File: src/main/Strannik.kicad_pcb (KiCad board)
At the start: 2 copper layers, 139 x 129 mm, 104 parts, among them J1 Thumb cluster, J2 Battery, SW1 Reset, SW11 SW_Push_Dual, SW12 SW_Push_Dual, SW13 SW_Push_Dual, SW14 SW_Push_Dual, SW15 SW_Push_Dual, SW16 SW_Push_Dual, SW17 SW_Push_Dual, SW21 SW_Push_Dual, SW22 SW_Push_Dual, SW23 SW_Push_Dual, SW24 SW_Push_Dual, SW25 SW_Push_Dual, SW26 SW_Push_Dual, SW27 SW_Push_Dual, SW31 SW_Push_Dual, SW32 SW_Push_Dual, SW33 SW_Push_Dual, SW34 SW_Push_Dual, SW35 SW_Push_Dual, SW36 SW_Push_Dual, SW37 SW_Push_Dual, SW41 SW_Push_Dual, SW42 SW_Push_Dual, SW43 SW_Push_Dual, SW44 SW_Push_Dual, SW45 SW_Push_Dual, SW46 SW_Push_Dual, SW51 SW_Push_Dual, SW52 SW_Push_Dual, SW53 SW_Push_Dual, SW54 SW_Push_Dual, SW55 SW_Push_Dual

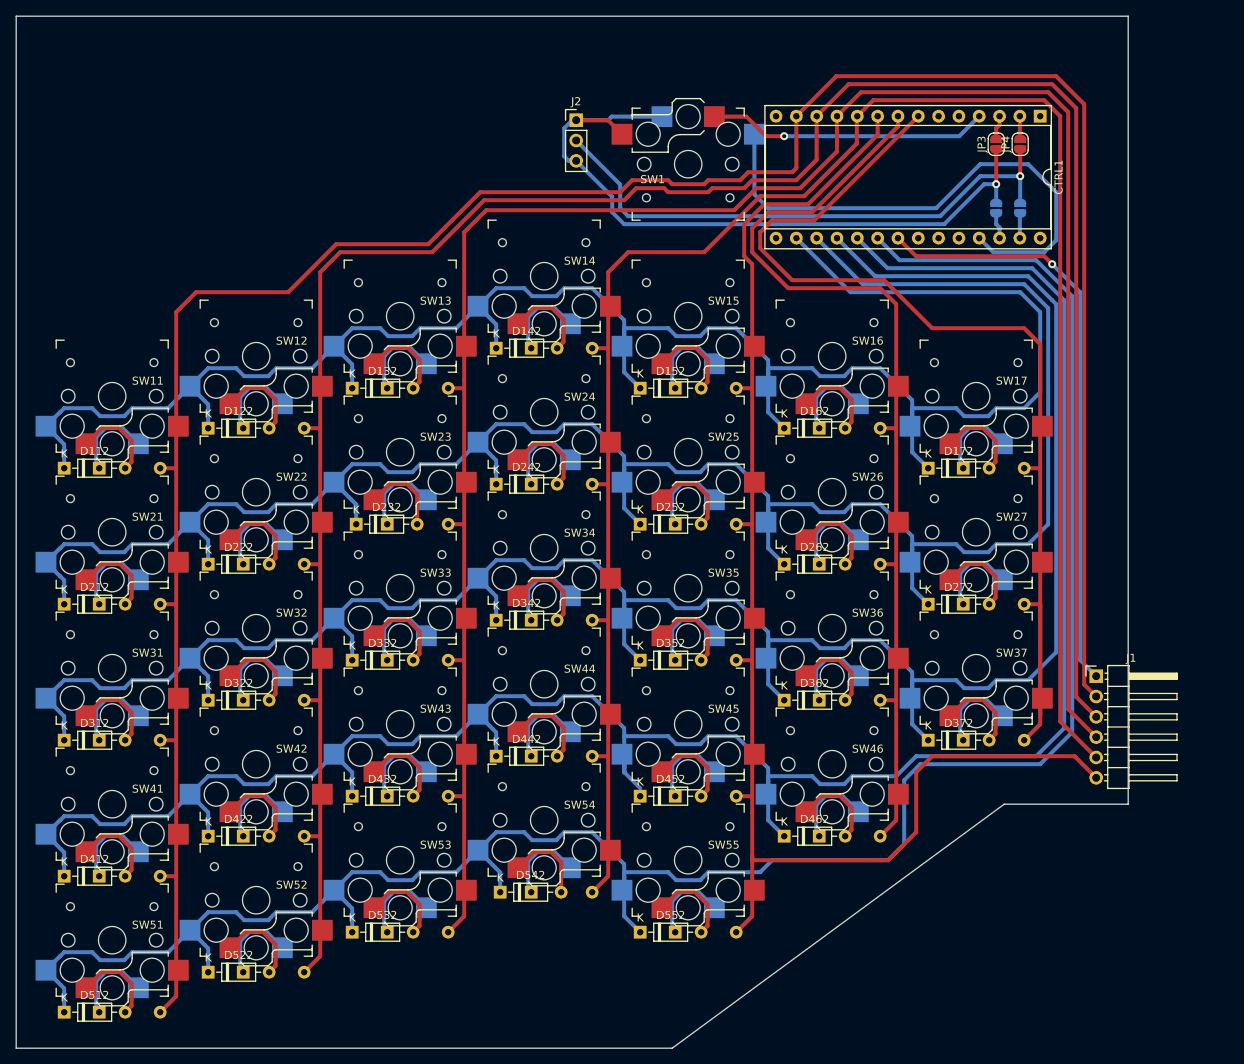
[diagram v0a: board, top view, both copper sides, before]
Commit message: new beautiful main board design
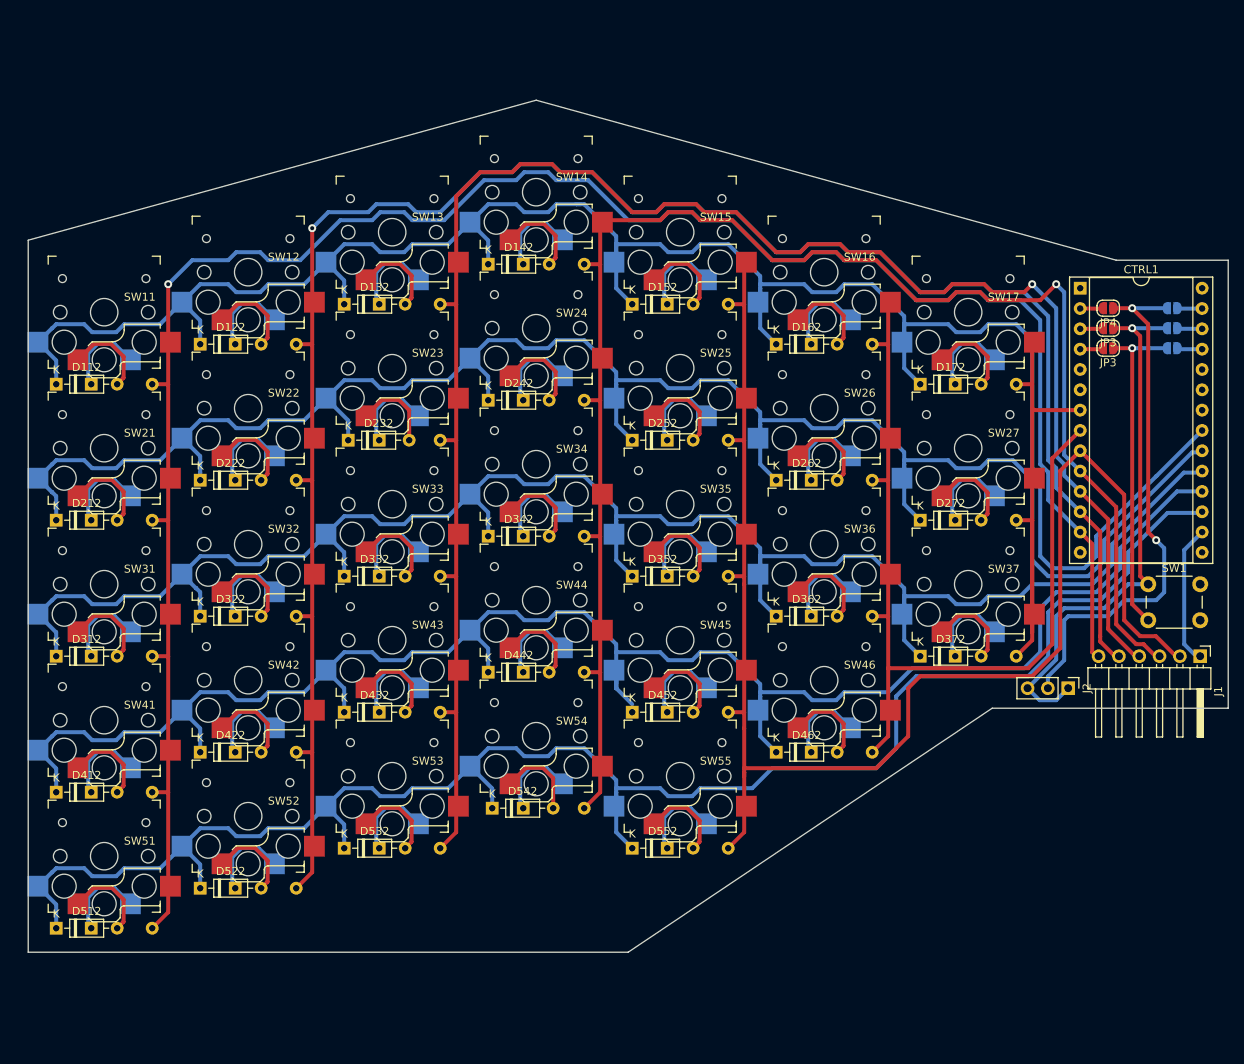
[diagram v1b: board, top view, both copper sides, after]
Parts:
- added JP1: Ground Left, Jumper:SolderJumper-2_P1.3mm_Open_RoundedPad1.0x1.5mm, B.Cu at (189.5, 76.5)
- added JP3: Ground Right, Jumper:SolderJumper-2_P1.3mm_Open_RoundedPad1.0x1.5mm, F.Cu at (181.5, 76.5)
- SW1: footprint Keyswitches:Kailh_socket_PG1350_reversible -> Button_Switch_THT:SW_PUSH_6mm_H4.3mm
- moved J2 93.9 mm to (176.5, 119.0), turned to -90 degrees
- moved SW1 77.9 mm to (186.5, 106.0), turned to 0 degrees
- moved JP3 26.9 mm to (181.5, 74.0), turned to 180 degrees
- moved JP1 26.6 mm to (189.5, 74.0), turned to 0 degrees
- moved JP4 23.3 mm to (181.5, 71.5), turned to 180 degrees
- moved JP2 22.7 mm to (189.5, 71.5), turned to 0 degrees
- moved CTRL1 22.1 mm to (178.0, 69.0), turned to 0 degrees
- moved J1 13.2 mm to (193.0, 115.0), turned to -90 degrees
- moved D111 10.5 mm to (54.4, 81.0)
- moved D112 10.5 mm to (50.0, 81.0)
- moved D121 10.5 mm to (72.4, 76.0)
- moved D122 10.5 mm to (68.0, 76.0)
- moved D131 10.5 mm to (90.4, 71.0)
- moved D132 10.5 mm to (86.0, 71.0)
- moved D141 10.5 mm to (108.4, 66.0)
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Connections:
- D112 pad 1: Net-(CTRL1-Pin_16) -> Net-(CTRL1-Pin_21)
- D122 pad 1: Net-(CTRL1-Pin_16) -> Net-(CTRL1-Pin_21)
- D132 pad 1: Net-(CTRL1-Pin_16) -> Net-(CTRL1-Pin_21)
- D142 pad 1: Net-(CTRL1-Pin_16) -> Net-(CTRL1-Pin_21)
- D152 pad 1: Net-(CTRL1-Pin_16) -> Net-(CTRL1-Pin_21)
- D162 pad 1: Net-(CTRL1-Pin_16) -> Net-(CTRL1-Pin_21)
- D172 pad 1: Net-(CTRL1-Pin_16) -> Net-(CTRL1-Pin_21)
- D212 pad 1: Net-(CTRL1-Pin_17) -> Net-(CTRL1-Pin_20)
- D222 pad 1: Net-(CTRL1-Pin_17) -> Net-(CTRL1-Pin_20)
- D232 pad 1: Net-(CTRL1-Pin_17) -> Net-(CTRL1-Pin_20)
- D242 pad 1: Net-(CTRL1-Pin_17) -> Net-(CTRL1-Pin_20)
- D252 pad 1: Net-(CTRL1-Pin_17) -> Net-(CTRL1-Pin_20)
- D262 pad 1: Net-(CTRL1-Pin_17) -> Net-(CTRL1-Pin_20)
- D272 pad 1: Net-(CTRL1-Pin_17) -> Net-(CTRL1-Pin_20)
- D312 pad 1: Net-(CTRL1-Pin_18) -> Net-(CTRL1-Pin_19)
- D322 pad 1: Net-(CTRL1-Pin_18) -> Net-(CTRL1-Pin_19)
- D332 pad 1: Net-(CTRL1-Pin_18) -> Net-(CTRL1-Pin_19)
- D342 pad 1: Net-(CTRL1-Pin_18) -> Net-(CTRL1-Pin_19)
- D352 pad 1: Net-(CTRL1-Pin_18) -> Net-(CTRL1-Pin_19)
- D362 pad 1: Net-(CTRL1-Pin_18) -> Net-(CTRL1-Pin_19)
- D372 pad 1: Net-(CTRL1-Pin_18) -> Net-(CTRL1-Pin_19)
- D412 pad 1: Net-(CTRL1-Pin_19) -> Net-(CTRL1-Pin_18)
- D422 pad 1: Net-(CTRL1-Pin_19) -> Net-(CTRL1-Pin_18)
- D432 pad 1: Net-(CTRL1-Pin_19) -> Net-(CTRL1-Pin_18)
- D442 pad 1: Net-(CTRL1-Pin_19) -> Net-(CTRL1-Pin_18)
- D452 pad 1: Net-(CTRL1-Pin_19) -> Net-(CTRL1-Pin_18)
- D462 pad 1: Net-(CTRL1-Pin_19) -> Net-(CTRL1-Pin_18)
- D512 pad 1: Net-(CTRL1-Pin_20) -> Net-(CTRL1-Pin_17)
- D522 pad 1: Net-(CTRL1-Pin_20) -> Net-(CTRL1-Pin_17)
- D532 pad 1: Net-(CTRL1-Pin_20) -> Net-(CTRL1-Pin_17)
- D542 pad 1: Net-(CTRL1-Pin_20) -> Net-(CTRL1-Pin_17)
- D552 pad 1: Net-(CTRL1-Pin_20) -> Net-(CTRL1-Pin_17)
- J1 pad 1: Net-(CTRL1-Pin_21) -> Net-(CTRL1-Pin_16)
- J1 pad 2: Net-(CTRL1-Pin_13) -> Net-(CTRL1-Pin_9)
- J1 pad 3: Net-(CTRL1-Pin_12) -> Net-(CTRL1-Pin_10)
- J1 pad 5: Net-(CTRL1-Pin_10) -> Net-(CTRL1-Pin_12)
- J1 pad 6: Net-(CTRL1-Pin_9) -> Net-(CTRL1-Pin_13)
- SW11 pad 2: Net-(CTRL1-Pin_16) -> Net-(CTRL1-Pin_21)
- SW12 pad 2: Net-(CTRL1-Pin_16) -> Net-(CTRL1-Pin_21)
- SW13 pad 2: Net-(CTRL1-Pin_16) -> Net-(CTRL1-Pin_21)
- SW14 pad 2: Net-(CTRL1-Pin_16) -> Net-(CTRL1-Pin_21)
- SW15 pad 2: Net-(CTRL1-Pin_16) -> Net-(CTRL1-Pin_21)
- SW16 pad 2: Net-(CTRL1-Pin_16) -> Net-(CTRL1-Pin_21)
- SW17 pad 2: Net-(CTRL1-Pin_16) -> Net-(CTRL1-Pin_21)
- SW21 pad 2: Net-(CTRL1-Pin_17) -> Net-(CTRL1-Pin_20)
- SW22 pad 2: Net-(CTRL1-Pin_17) -> Net-(CTRL1-Pin_20)
- SW23 pad 2: Net-(CTRL1-Pin_17) -> Net-(CTRL1-Pin_20)
- SW24 pad 2: Net-(CTRL1-Pin_17) -> Net-(CTRL1-Pin_20)
- SW25 pad 2: Net-(CTRL1-Pin_17) -> Net-(CTRL1-Pin_20)
- SW26 pad 2: Net-(CTRL1-Pin_17) -> Net-(CTRL1-Pin_20)
- SW27 pad 2: Net-(CTRL1-Pin_17) -> Net-(CTRL1-Pin_20)
- SW31 pad 2: Net-(CTRL1-Pin_18) -> Net-(CTRL1-Pin_19)
- SW32 pad 2: Net-(CTRL1-Pin_18) -> Net-(CTRL1-Pin_19)
- SW33 pad 2: Net-(CTRL1-Pin_18) -> Net-(CTRL1-Pin_19)
- SW34 pad 2: Net-(CTRL1-Pin_18) -> Net-(CTRL1-Pin_19)
- SW35 pad 2: Net-(CTRL1-Pin_18) -> Net-(CTRL1-Pin_19)
- SW36 pad 2: Net-(CTRL1-Pin_18) -> Net-(CTRL1-Pin_19)
- SW37 pad 2: Net-(CTRL1-Pin_18) -> Net-(CTRL1-Pin_19)
- SW41 pad 2: Net-(CTRL1-Pin_19) -> Net-(CTRL1-Pin_18)
- SW42 pad 2: Net-(CTRL1-Pin_19) -> Net-(CTRL1-Pin_18)
- SW43 pad 2: Net-(CTRL1-Pin_19) -> Net-(CTRL1-Pin_18)
- SW44 pad 2: Net-(CTRL1-Pin_19) -> Net-(CTRL1-Pin_18)
- SW45 pad 2: Net-(CTRL1-Pin_19) -> Net-(CTRL1-Pin_18)
- SW46 pad 2: Net-(CTRL1-Pin_19) -> Net-(CTRL1-Pin_18)
- SW51 pad 2: Net-(CTRL1-Pin_20) -> Net-(CTRL1-Pin_17)
- SW52 pad 2: Net-(CTRL1-Pin_20) -> Net-(CTRL1-Pin_17)
- SW53 pad 2: Net-(CTRL1-Pin_20) -> Net-(CTRL1-Pin_17)
- SW54 pad 2: Net-(CTRL1-Pin_20) -> Net-(CTRL1-Pin_17)
- SW55 pad 2: Net-(CTRL1-Pin_20) -> Net-(CTRL1-Pin_17)
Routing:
- net Net-(CTRL1-Pin_16): track 247.3 -> 17.1 mm
- net Net-(CTRL1-Pin_21): track 74.4 -> 259.9 mm, vias 1 -> 0
- net Net-(CTRL1-Pin_7): track 136.1 -> 64.3 mm
- net Net-(CTRL1-Pin_18): track 279.4 -> 227.9 mm
- net Net-(CTRL1-Pin_19): track 279.6 -> 230.8 mm
- net Net-(CTRL1-Pin_17): track 262.4 -> 217.5 mm
- net Net-(CTRL1-Pin_13): track 302.4 -> 260.8 mm, vias 0 -> 1
- net Net-(CTRL1-Pin_12): track 282.5 -> 243.8 mm, vias 0 -> 1
- net Net-(CTRL1-Pin_10): track 236.6 -> 198.7 mm, vias 0 -> 1
- net Net-(CTRL1-Pin_11): track 262.3 -> 225.3 mm, vias 0 -> 1
- net Net-(CTRL1-Pin_4): track 35.2 -> 2.90 mm, vias 1 -> 0
- net Net-(CTRL1-Pin_20): track 271.2 -> 241.9 mm
- net Net-(CTRL1-Pin_25): track 66.7 -> 44.7 mm, vias 0 -> 1
- net Net-(J2-Pin_1): track 90.3 -> 69.5 mm
- net Net-(CTRL1-Pin_9): track 175.8 -> 189.4 mm
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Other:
- board size 139 x 129 mm -> 150 x 106.5 mm
